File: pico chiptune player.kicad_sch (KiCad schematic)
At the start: 24 parts, among them J1 MicroSD, J2 Speaker Out, SW1 Play / Pause, SW2 Next, SW3 Previous, U1 AY-3-8910, U2 PAM8302AAS, U3 0.96"OLED_I2C

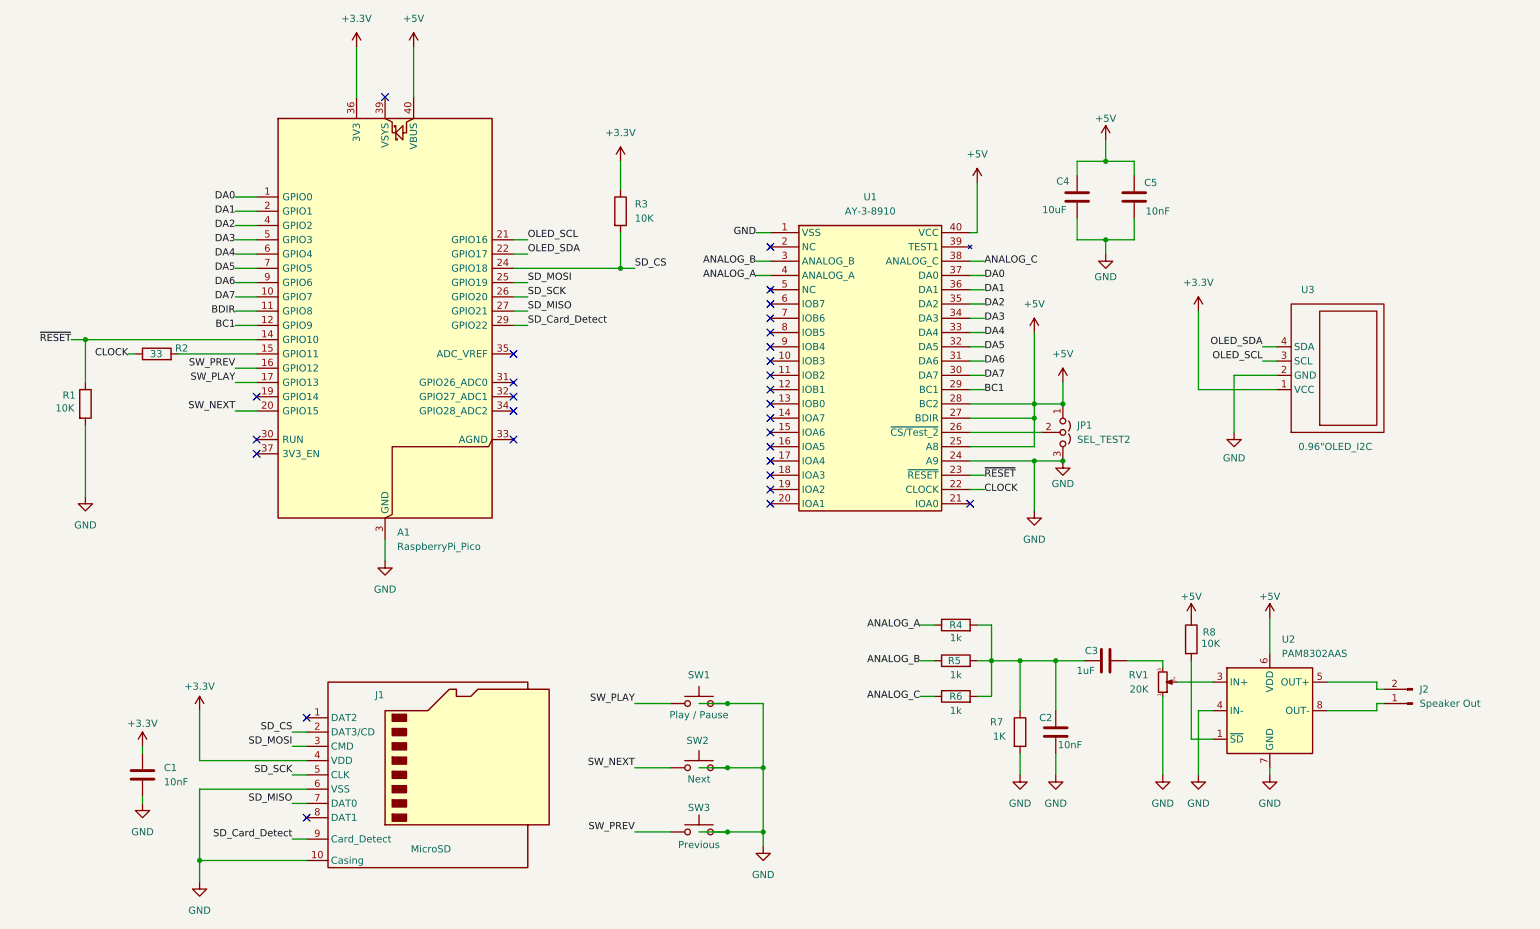
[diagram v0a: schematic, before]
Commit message: Refactor code structure for improved readability and maintainability
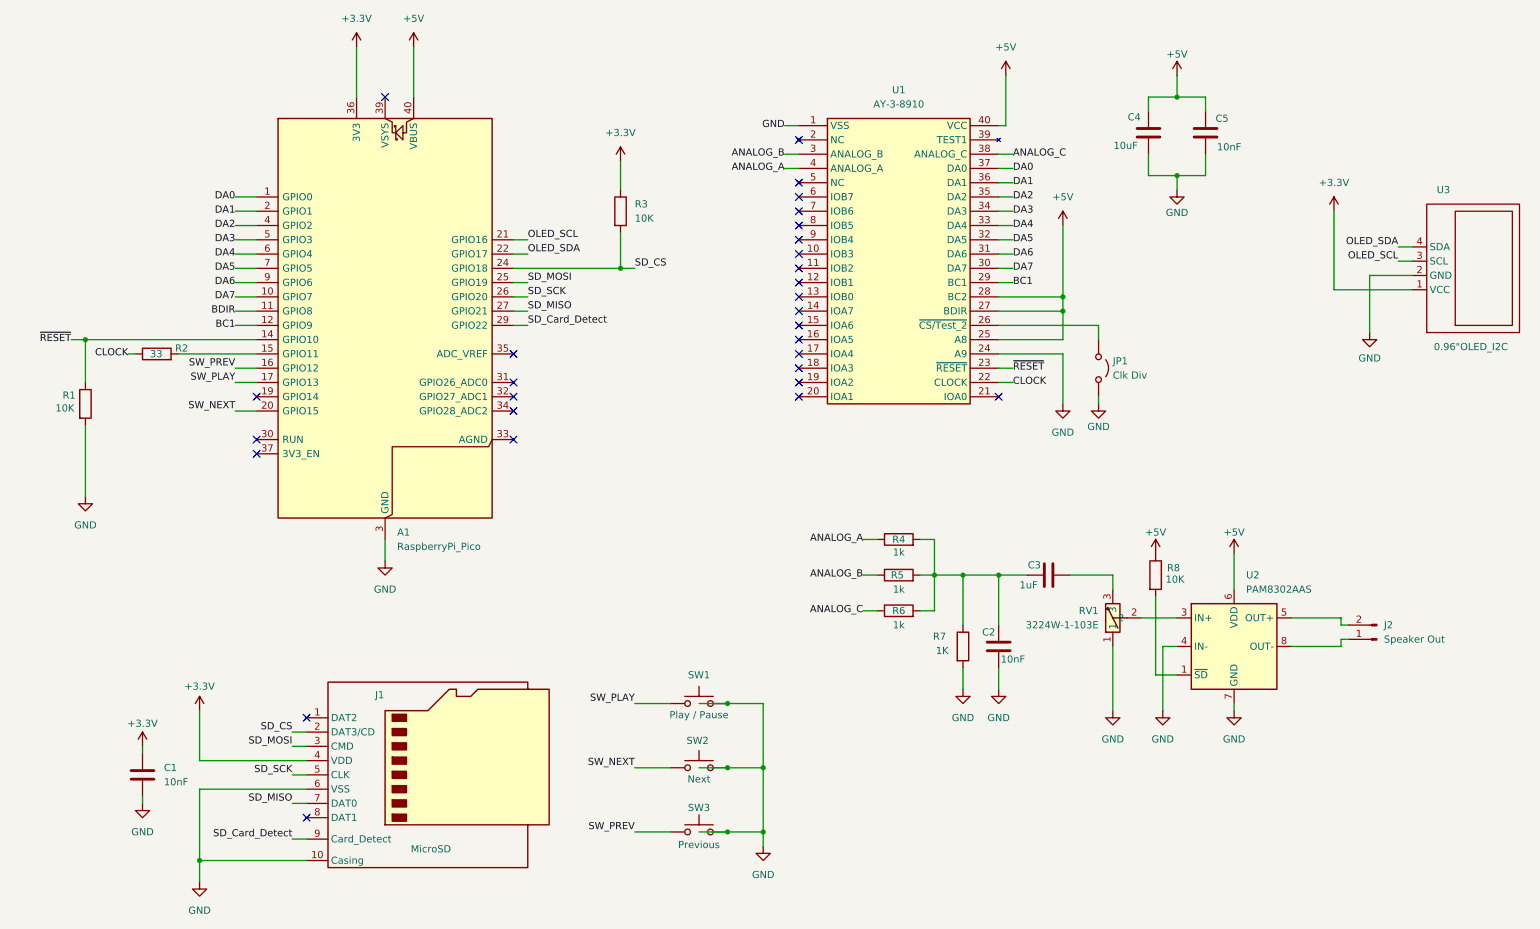
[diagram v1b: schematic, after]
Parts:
- removed JP1: SEL_TEST2, Jumper:SolderJumper-3_P2.0mm_Open_TrianglePad1.0x1.5mm, symbol Jumper:Jumper_3_Open
- removed RV1: 20K, symbol Device:R_Potentiometer_Small
- added JP1: Clk Div, Jumper:SolderJumper-2_P1.3mm_Open_TrianglePad1.0x1.5mm, symbol Jumper:Jumper_2_Open
- added RV1: 3224W-1-103E, Potentiometer_SMD:Potentiometer_Bourns_3224W_Vertical, symbol BOURNS_3224W-1-103E:BOURNS_3224W-1-103E
- U2: footprint (none) -> Package_SO:SOIC-8_5.3x5.3mm_P1.27mm
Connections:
- net GND: now also JP1.2 (B), RV1.1
- net at U1.26 (~{CS/Test_2}): now also JP1.1 (A)
- net at U2.3 (IN+): now also RV1.2
- net at C3.2: now also RV1.3
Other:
- moved on the sheet: C2, C3, C4, C5, J2, R4, R5, R6, R7, R8, U1, U2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
